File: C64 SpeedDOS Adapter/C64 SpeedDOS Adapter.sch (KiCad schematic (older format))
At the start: 6 parts, among them J1 C64_User_Port, J2 SpeedDOS, M1 Mounting, M2 Mounting, M3 Mounting, M4 Mounting

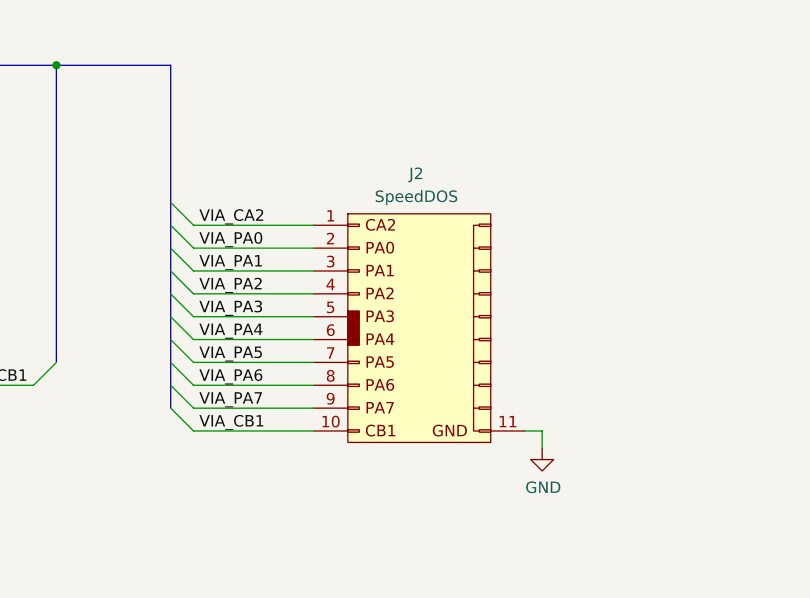
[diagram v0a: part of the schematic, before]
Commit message: Updated gerber files and small tweaks
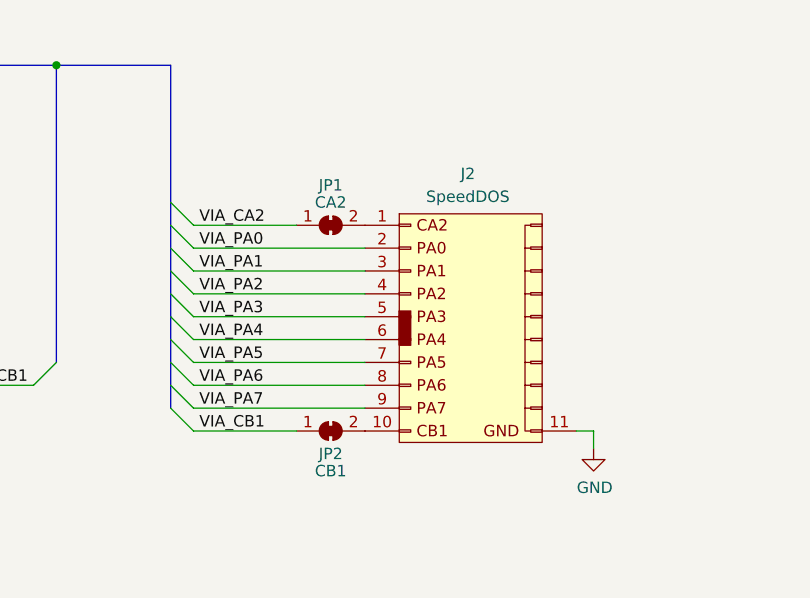
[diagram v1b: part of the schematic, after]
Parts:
- added JP1: CA2, solder_bridge:bridge, symbol Jumper:SolderJumper_2_Bridged
- added JP2: CB1, solder_bridge:bridge_r, symbol Jumper:SolderJumper_2_Bridged
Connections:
- net VIA_CA2: now also JP1.1 (A); no longer J2.1 (Pin_1)
- net VIA_CB1: now also JP2.1 (A); no longer J2.10 (Pin_10)
- new net: J2.1 (Pin_1), JP1.2 (B)
- new net: J2.10 (Pin_10), JP2.2 (B)
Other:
- moved on the sheet: J2
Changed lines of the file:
@@
 L speed_dos:Speed_DOS_IDC J2
 U 1 1 5EF167B3
-P 7975 2700
-F 0 "J2" H 7975 3125 50  0000 C CNN
-F 1 "SpeedDOS" H 7975 3025 50  0000 C CNN
-F 2 "speed_dos:SpeedDOS_IDC" H 7975 2700 50  0001 C CNN
-F 3 "~" H 7975 2700 50  0001 C CNN
-	1    7975 2700
+P 8200 2700
+F 0 "J2" H 8200 3125 50  0000 C CNN
+F 1 "SpeedDOS" H 8200 3025 50  0000 C CNN
+F 2 "speed_dos:SpeedDOS_IDC" H 8200 2700 50  0001 C CNN
+F 3 "~" H 8200 2700 50  0001 C CNN
+	1    8200 2700
 	1    0    0    -1
 $EndComp
@@
 L power:GND #PWR01
 U 1 1 5EF2A7F5
-P 8525 3475
-F 0 "#PWR01" H 8525 3225 50  0001 C CNN
-F 1 "GND" H 8530 3302 50  0000 C CNN
-F 2 "" H 8525 3475 50  0001 C CNN
-F 3 "" H 8525 3475 50  0001 C CNN
-	1    8525 3475
-	1    0    0    -1
-$EndComp
-Wire Wire Line
-	8450 3400 8525 3400
-Wire Wire Line
-	8525 3400 8525 3475
+P 8750 3475
+F 0 "#PWR01" H 8750 3225 50  0001 C CNN
+F 1 "GND" H 8755 3302 50  0000 C CNN
+F 2 "" H 8750 3475 50  0001 C CNN
+F 3 "" H 8750 3475 50  0001 C CNN
+	1    8750 3475
+	1    0    0    -1
+$EndComp
+Wire Wire Line
+	8675 3400 8750 3400
+Wire Wire Line
+	8750 3400 8750 3475
 Text Label 7025 2600 0    50   ~ 0
 VIA_PA0
@@
 VIA_CB1
 Wire Wire Line
-	7000 2500 7525 2500
-Wire Wire Line
-	7525 2600 7000 2600
-Wire Wire Line
-	7000 2700 7525 2700
-Wire Wire Line
-	7000 2800 7525 2800
-Wire Wire Line
-	7525 2900 7000 2900
-Wire Wire Line
-	7000 3000 7525 3000
-Wire Wire Line
-	7000 3100 7525 3100
-Wire Wire Line
-	7525 3200 7000 3200
-Wire Wire Line
-	7000 3300 7525 3300
-Wire Wire Line
-	7000 3400 7525 3400
+	7000 2500 7450 2500
 $Comp
 L C64-User-Port:C64_User_Port J1
@@
 	1    0    0    -1
 $EndComp
+$Comp
+L Jumper:SolderJumper_2_Bridged JP1
+U 1 1 60764DE4
+P 7600 2500
+F 0 "JP1" H 7600 2675 50  0000 C CNN
+F 1 "CA2" H 7600 2600 50  0000 C CNN
+F 2 "solder_bridge:bridge" H 7600 2500 50  0001 C CNN
+F 3 "~" H 7600 2500 50  0001 C CNN
+	1    7600 2500
+	1    0    0    -1
+$EndComp
+$Comp
+L Jumper:SolderJumper_2_Bridged JP2
+U 1 1 6077FA79
+P 7600 3400
+F 0 "JP2" H 7600 3300 50  0000 C CNN
+F 1 "CB1" H 7600 3225 50  0000 C CNN
+F 2 "solder_bridge:bridge_r" H 7600 3400 50  0001 C CNN
+F 3 "~" H 7600 3400 50  0001 C CNN
+	1    7600 3400
+	1    0    0    -1
+$EndComp
+Wire Wire Line
+	7000 2600 7750 2600
+Wire Wire Line
+	7000 2700 7750 2700
+Wire Wire Line
+	7000 2800 7750 2800
+Wire Wire Line
+	7000 2900 7750 2900
+Wire Wire Line
+	7000 3000 7750 3000
+Wire Wire Line
+	7000 3100 7750 3100
+Wire Wire Line
+	7000 3200 7750 3200
+Wire Wire Line
+	7000 3300 7750 3300
+Wire Wire Line
+	7450 3400 7000 3400
+Wire Bus Line
+	6900 1800 6900 3300
 Wire Bus Line
 	3850 1800 3850 3300
-Wire Bus Line
-	6900 1800 6900 3300
 $EndSCHEMATC
